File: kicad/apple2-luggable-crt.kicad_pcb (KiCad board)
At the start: 2 copper layers, 145.3 x 120.3 mm, 241 parts, among them J1 VIDEO IN, J401 DEFLECTION YOKE, J402 CRT SOCKET BRD, J403 PICTURE CONTROLS, J404 PICTURE CONTROLS, J501 CRT SOCKET BRD, J801 12V UNREG, Q201 2SA562-Y, Q202 2SC1815-Y, Q301 2SC2236A-Y, Q302 2SC2236A-Y, Q303 2SC1815-Y, Q304 2SA1015-Y, Q401 2SC200-Y, Q402 2SC2233, Q501 TD7698AP, SW201 SW_SP3T, T401 L_Ferrite_Coupled_1243, T451 KFB-2007 / 8D04K, T502 KRFE204, U1 XRP29302ETBTR-L, X501 3.579545MHz

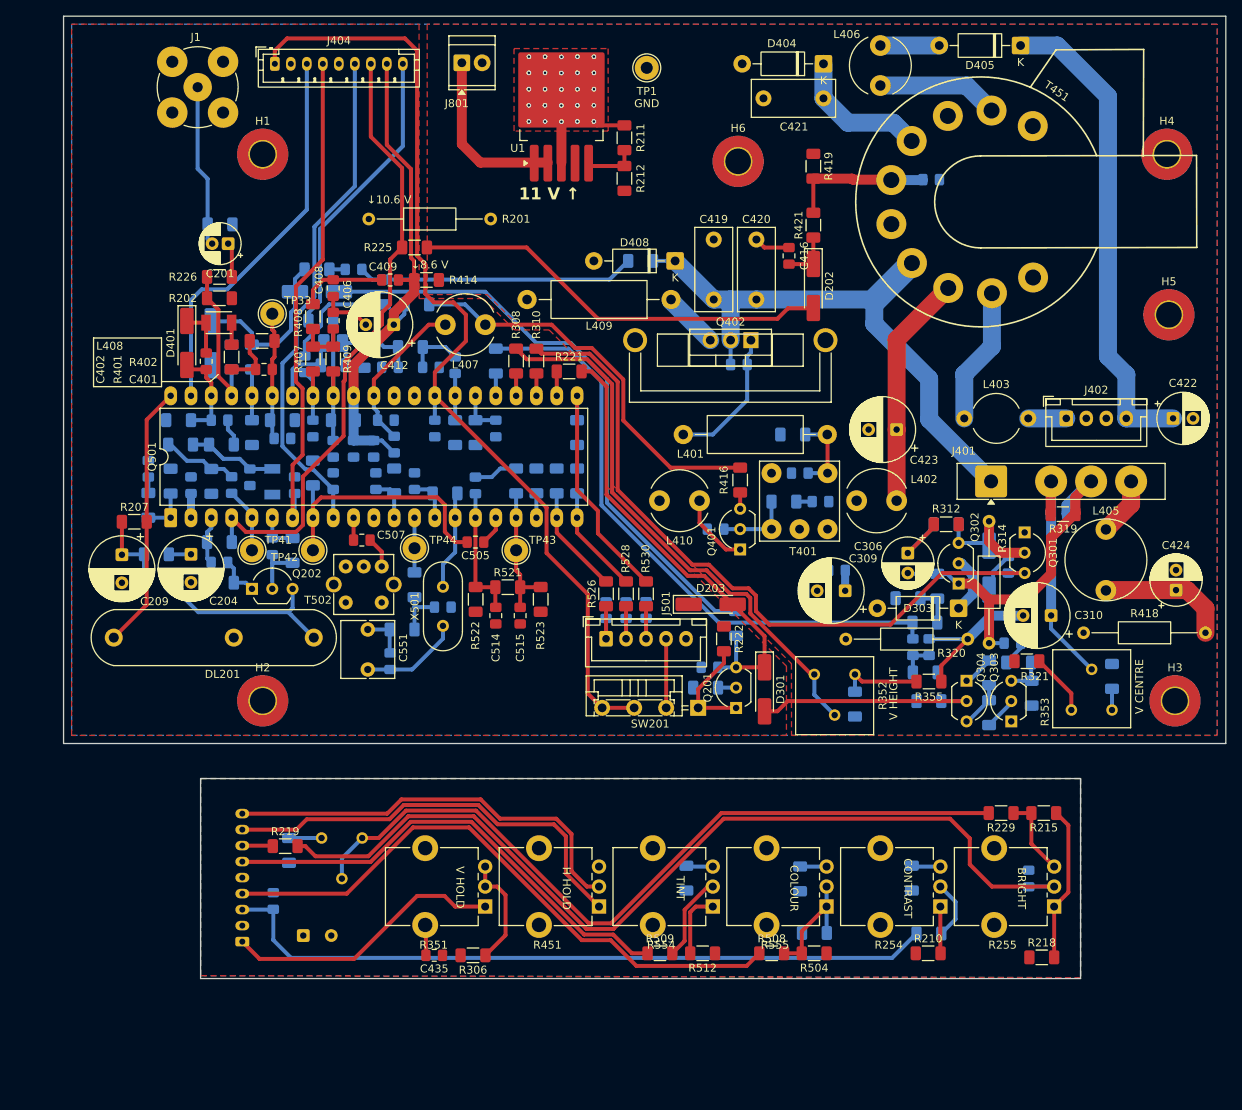
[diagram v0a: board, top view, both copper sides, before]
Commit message: version before heat sink work
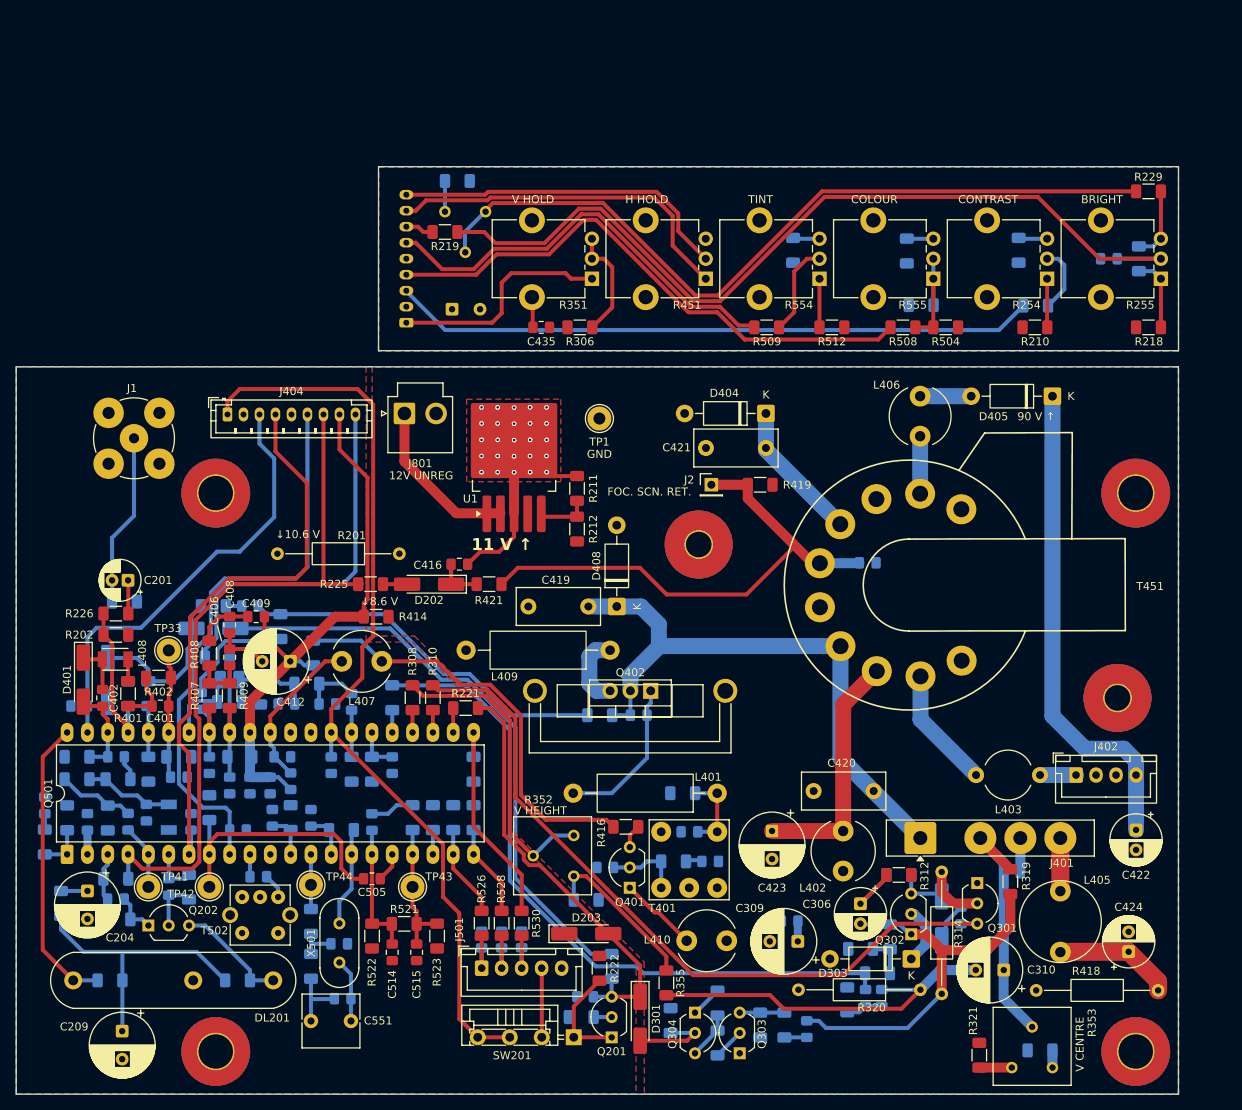
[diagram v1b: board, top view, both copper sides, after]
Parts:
- added J2: FOC. SCN. RET., Connector_PinHeader_2.54mm:PinHeader_1x01_P2.54mm_Vertical, F.Cu at (136.2, 77.9)
- C507, R207, R215: moved to B.Cu
- H1, H2, H3, H4: value M3 -> M4; footprint MountingHole:MountingHole_3.2mm_M3_Pad_TopBottom -> MountingHole:MountingHole_4.3mm_M4_Pad_TopBottom
- H5, H6: footprint MountingHole:MountingHole_3.2mm_M3_Pad_TopBottom -> foodprints:MountingHole_3.2mm_M3_Pad_TopBottom_flyback_shield
- J801: footprint TerminalBlock_TE-Connectivity:TerminalBlock_TE_282834-2_1x02_P2.54mm_Horizontal -> Connector_JST:JST_VH_B2P-VH_1x02_P3.96mm_Vertical
- moved R230 86.3 mm to (104.4, 39.9), turned to 0 degrees
- moved C210 80.5 mm to (103.7, 55.9)
- moved J403 80.0 mm to (98.0, 57.6)
- moved R504 80.0 mm to (165.5, 58.2)
- moved R508 79.9 mm to (160.1, 58.2)
- moved R512 79.9 mm to (151.2, 58.2)
- moved R218 79.9 mm to (190.8, 58.2)
- moved R229 79.9 mm to (190.8, 41.2)
- moved R257 79.8 mm to (107.9, 43.8)
- moved C435 79.6 mm to (114.9, 58.2)
- moved R306 79.6 mm to (119.7, 58.2)
- moved R213 79.6 mm to (174.6, 48.6)
- moved R214 79.6 mm to (176.7, 55.5)
- moved R507 79.6 mm to (160.6, 48.7)
- moved R515 79.6 mm to (146.4, 48.6)
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- renumbered RV14 to R129
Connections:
- net Net-(D405-K) renamed /90V
- net Net-(J402-Pin_1) renamed /HEATER ACV
- net Net-(J801-Pin_1) renamed /12 V UNREG
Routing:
- net Net-(D202-A): track 52.5 -> 2.55 mm
- net Net-(J2-Pin_1): track 18.7 -> 65.1 mm
- net Net-(R308-Pad2): track 69.3 -> 38.3 mm
- net Net-(C310-Pad2): track 19.7 -> 46.2 mm
- net Net-(C209-Pad1): track 10.4 -> 34.5 mm
- net /VERT BLANKING: track 28.9 -> 10.3 mm
- net /V HOLD: track 159.2 -> 145.5 mm
- net /H. PULSE: track 34.8 -> 46.8 mm
- net Net-(R352-Pad3): track 10.2 -> 20.5 mm
- net Net-(R215-Pad1): track 19.4 -> 9.22 mm
- net Net-(Q202-B): track 24.1 -> 14.1 mm
- net /BRIGHT: track 81.4 -> 90.8 mm
- net Net-(C308-Pad1): track 77.7 -> 87.0 mm
- net Net-(C208-Pad1): track 117.4 -> 109.1 mm
- net Net-(L406-Pad1): track 15.2 -> 7.19 mm
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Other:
- board size 145.3 x 120.3 mm -> 145.3 x 115.9 mm
- board text added: "https://github.com/cannon-zz/luggable-colour-crt-monitor.git"
